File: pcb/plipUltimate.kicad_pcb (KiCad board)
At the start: 2 copper layers, 50 x 50 mm, 51 parts, among them CON1 IEEEE-1284A, CON2 AVR-ISP-6, CON3 RJ45_C, CON4 USB_microB, CON5 SD_SPI, U1 ENC28J60, U2 ATMEGA328P, U3 LM2596_5.0, U4 74LVC125, U5 IRF7309, U6 IRF7309, U7 AMS1117_3V3, X1 25MHz

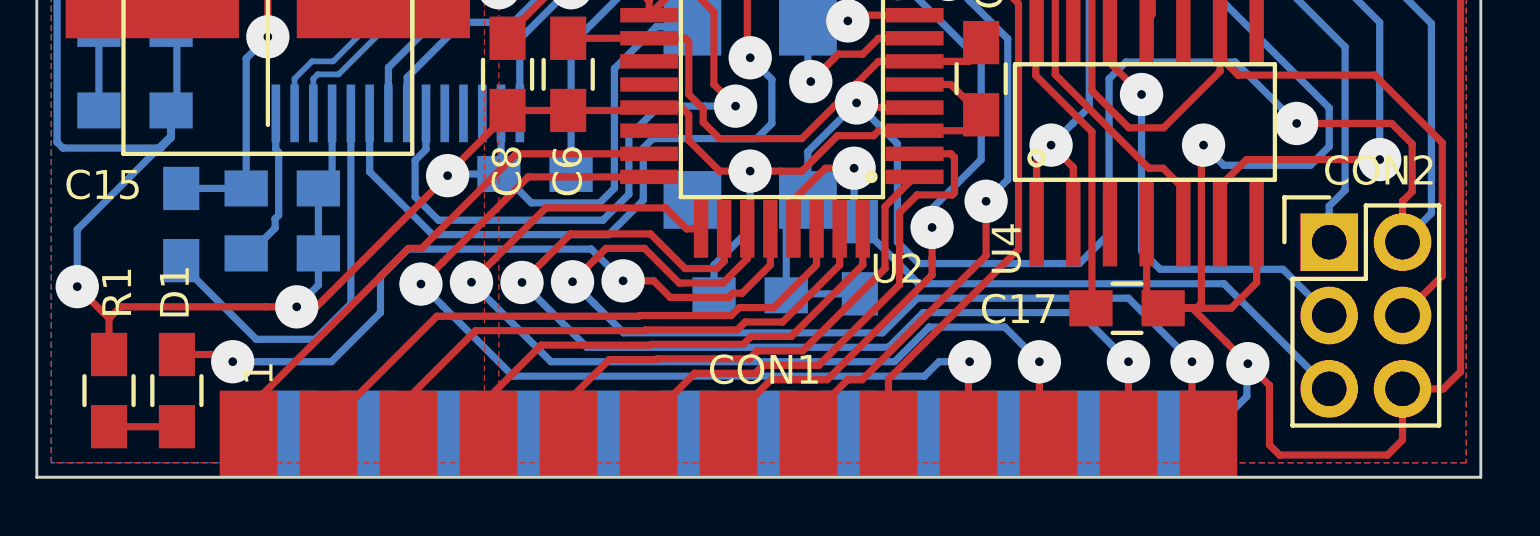
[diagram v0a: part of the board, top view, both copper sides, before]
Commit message: minor layout tweaks
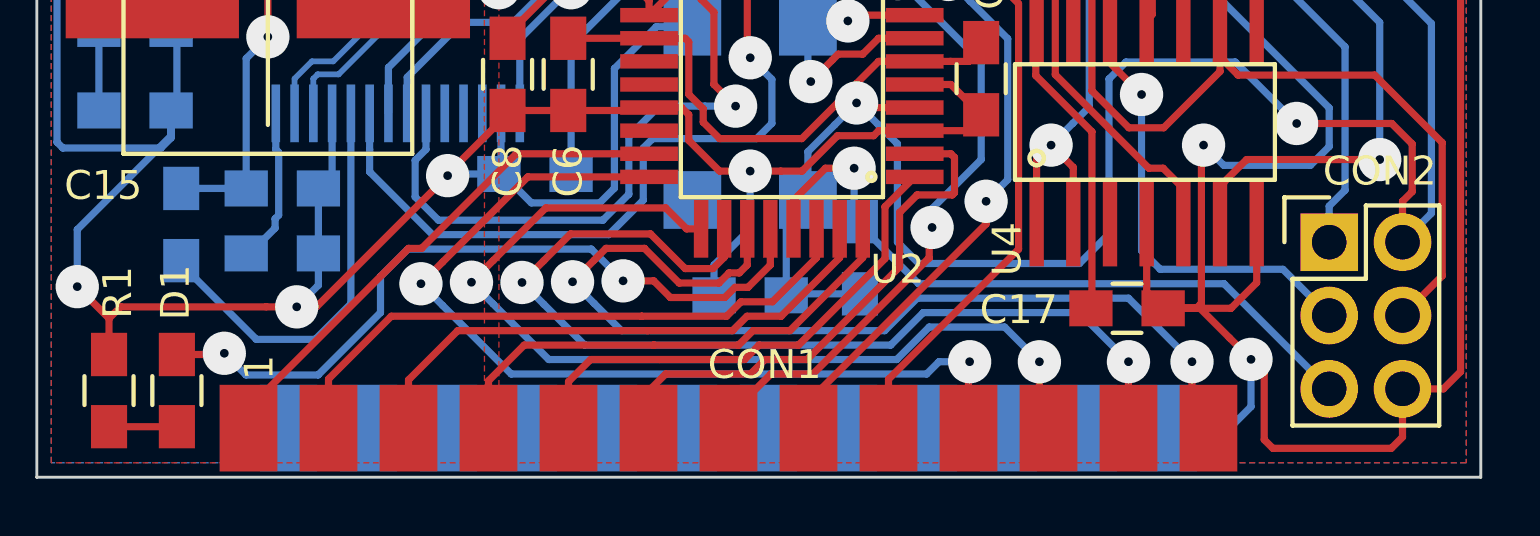
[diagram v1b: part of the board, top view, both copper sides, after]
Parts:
- moved CON1 0.20 mm to (57.3, 133.3)
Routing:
- net GND: track 465.9 -> 468.3 mm
- net /D0: track 21.3 -> 22.0 mm
